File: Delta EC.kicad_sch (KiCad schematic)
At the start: 42 parts, among them J1 USB_C_Receptacle_USB2.0_16P, J2 Conn_01x08, J3 Conn_01x18, J4 Conn_01x18, U1 STM32G474CBTx, U2 USBLC6-2SC6, U3 TPS7A2033, Y1 8Mhz 12pF

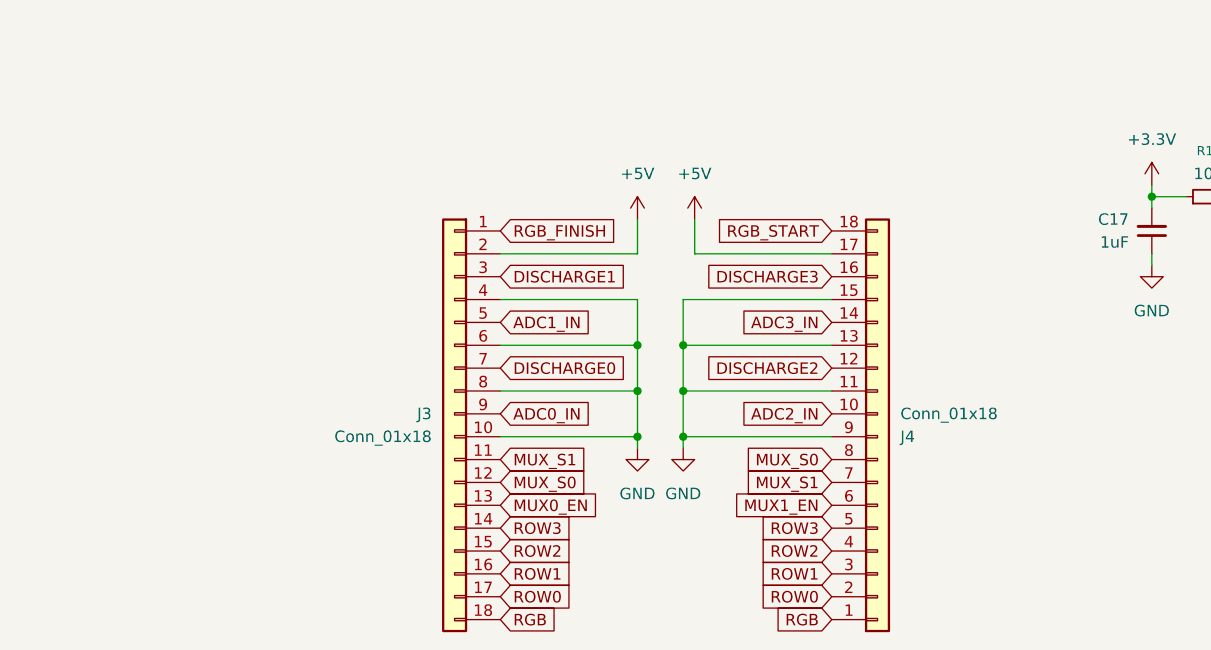
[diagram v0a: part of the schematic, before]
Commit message: 16.04.2026
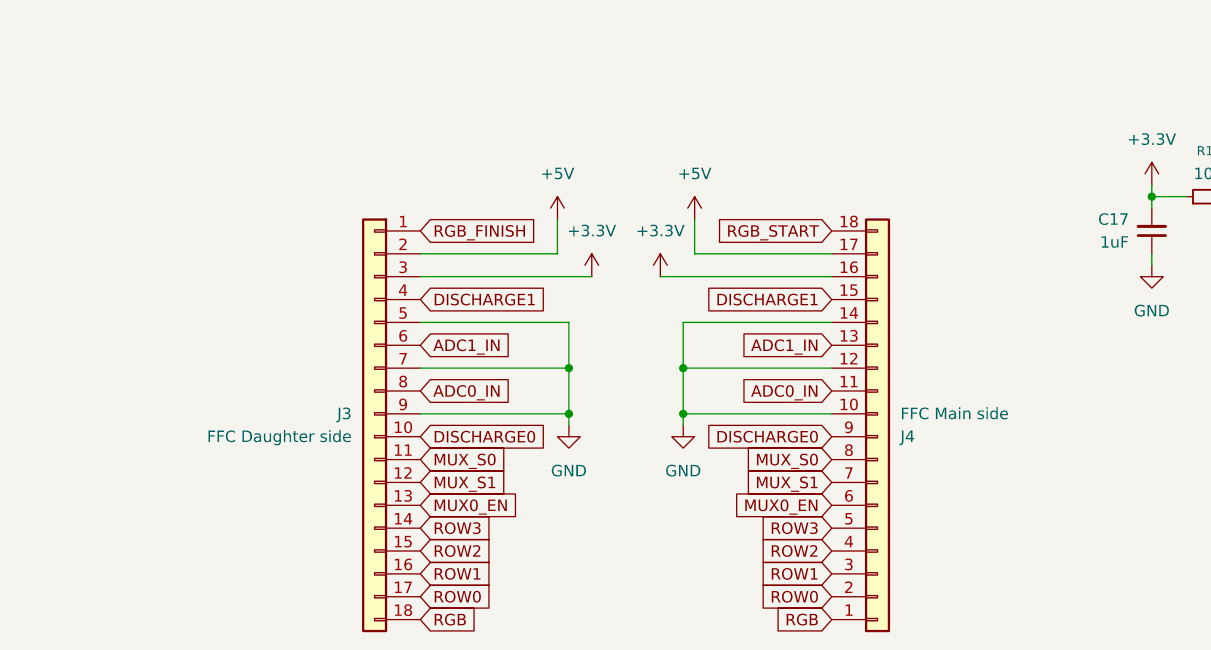
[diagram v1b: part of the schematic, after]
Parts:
- J3: value Conn_01x18 -> FFC Daughter side
- J4: value Conn_01x18 -> FFC Main side
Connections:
- net +3.3V: now also J3.3 (Pin_3), J4.16 (Pin_16)
- net ADC0_IN: now also J3.8 (Pin_8), J4.11 (Pin_11); no longer J3.9 (Pin_9)
- net ADC1_IN: now also J3.6 (Pin_6), J4.13 (Pin_13); no longer J3.5 (Pin_5)
- net ADC2_IN: no longer J4.10 (Pin_10)
- net ADC3_IN: no longer J4.14 (Pin_14)
- net DISCHARGE0: now also J3.10 (Pin_10), J4.9 (Pin_9); no longer J3.7 (Pin_7)
- net DISCHARGE1: now also J3.4 (Pin_4), J4.15 (Pin_15); no longer J3.3 (Pin_3)
- net DISCHARGE2: no longer J4.12 (Pin_12)
- net DISCHARGE3: no longer J4.16 (Pin_16)
- net GND: now also J3.5 (Pin_5), J3.7 (Pin_7), J3.9 (Pin_9), J4.10 (Pin_10), J4.12 (Pin_12), J4.14 (Pin_14); no longer J3.10 (Pin_10), J3.4 (Pin_4), J3.6 (Pin_6), J3.8 (Pin_8), J4.11 (Pin_11), J4.13 (Pin_13), J4.15 (Pin_15), J4.9 (Pin_9)
- net MUX0_EN: now also J4.6 (Pin_6)
- net MUX1_EN: no longer J4.6 (Pin_6)
- net MUX_S0: now also J3.11 (Pin_11); no longer J3.12 (Pin_12)
- net MUX_S1: now also J3.12 (Pin_12); no longer J3.11 (Pin_11)
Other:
- moved on the sheet: J3

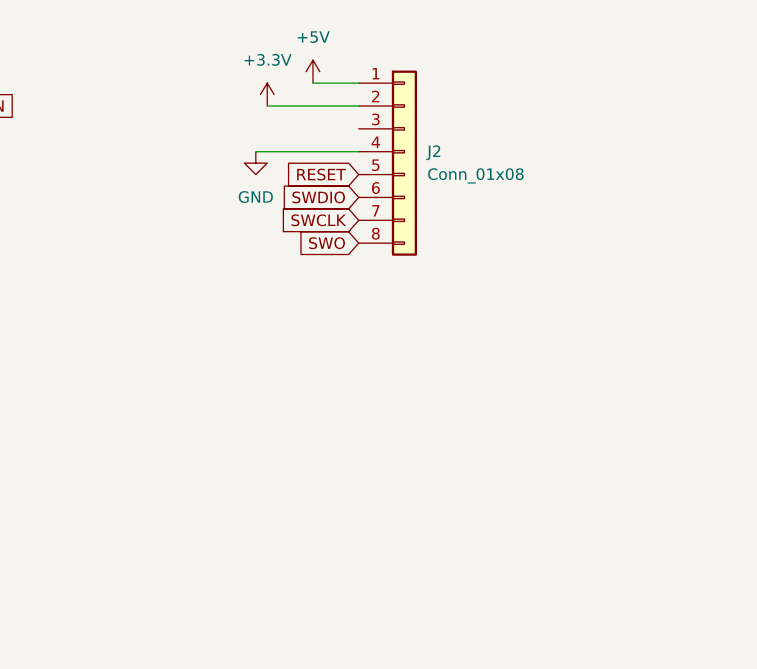
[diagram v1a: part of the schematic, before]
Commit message: 16.04.2026
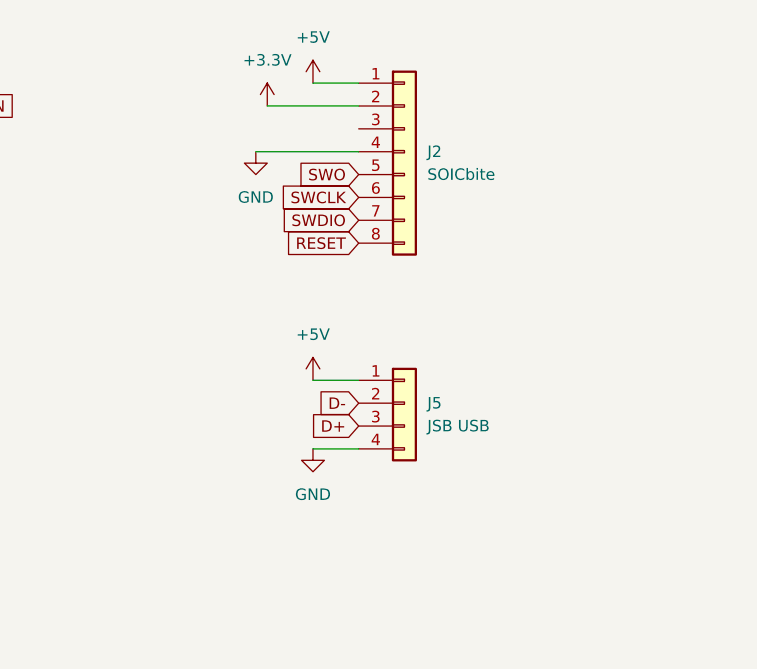
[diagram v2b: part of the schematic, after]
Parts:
- added J5: JSB USB, Connector_JST:JST_SH_SM04B-SRSS-TB_1x04-1MP_P1.00mm_Horizontal, symbol Connector_Generic:Conn_01x04
- J2: value Conn_01x08 -> SOICbite
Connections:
- net +5V: now also J5.1 (Pin_1)
- net D+: now also J5.3 (Pin_3)
- net D-: now also J5.2 (Pin_2)
- net GND: now also J5.4 (Pin_4)
- net RESET: now also J2.8 (Pin_8); no longer J2.5 (Pin_5)
- net SWCLK: now also J2.6 (Pin_6); no longer J2.7 (Pin_7)
- net SWDIO: now also J2.7 (Pin_7); no longer J2.6 (Pin_6)
- net SWO: now also J2.5 (Pin_5); no longer J2.8 (Pin_8)
